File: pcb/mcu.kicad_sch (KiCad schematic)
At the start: 34 parts, among them J1 Conn_01x02_Pin, SW1 SW_SPDT, SW2 SW_Push, SW3 SW_SPDT, U1 TLV1117LV33DCYR, U2 W25Q64JVSSIQ_C179171, U3 STM32H750VBTx, Y1 25 MHz

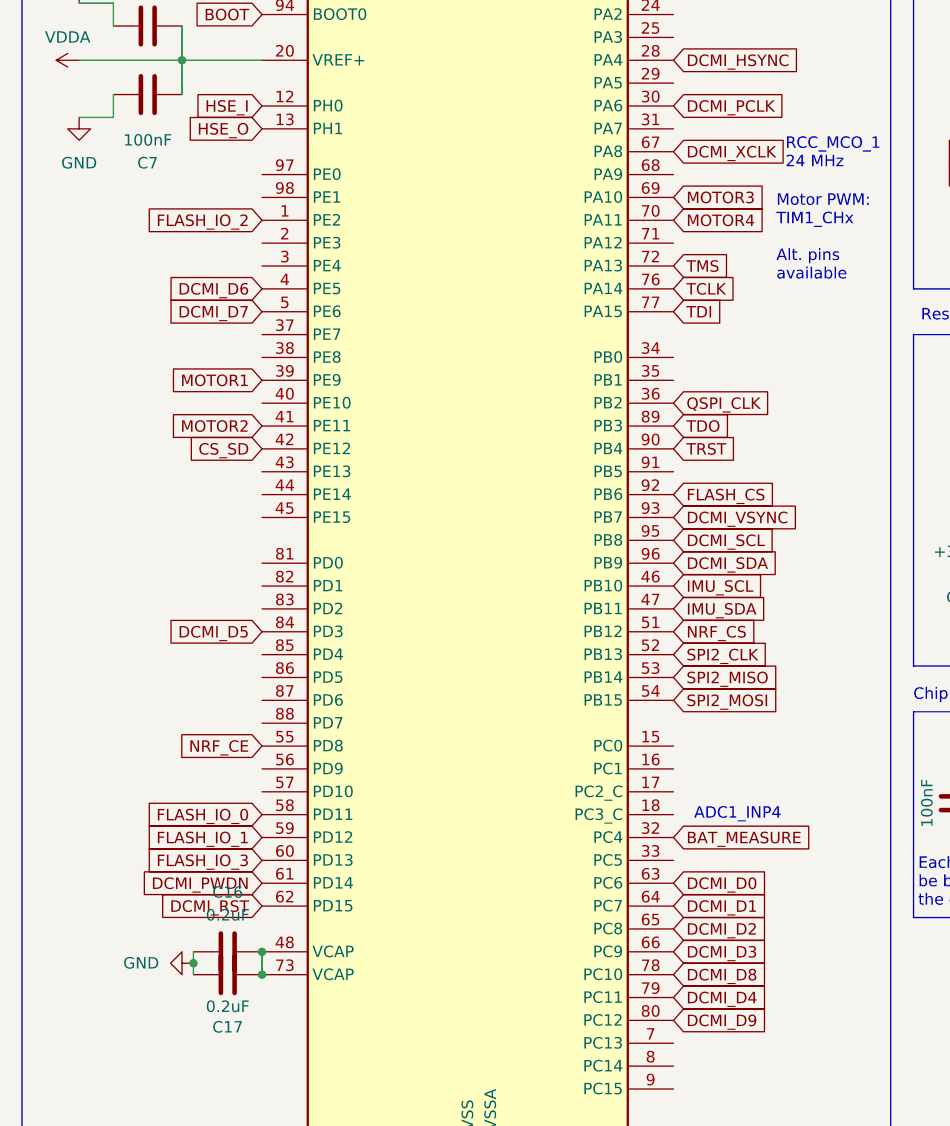
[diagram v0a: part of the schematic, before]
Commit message: [pcb] more routing
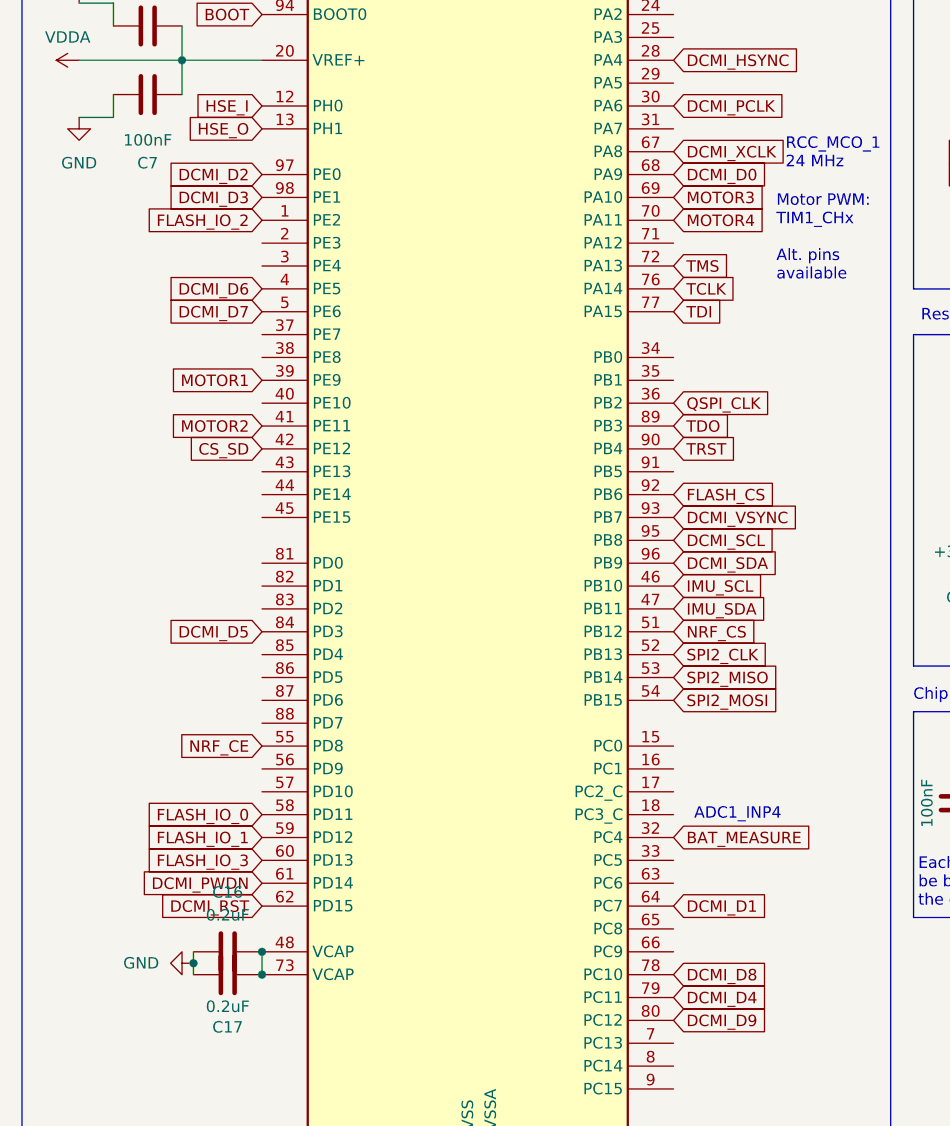
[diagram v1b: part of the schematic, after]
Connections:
- net DCMI_D0: now also U3.68 (PA9); no longer U3.63 (PC6)
- net DCMI_D2: now also U3.97 (PE0); no longer U3.65 (PC8)
- net DCMI_D3: now also U3.98 (PE1); no longer U3.66 (PC9)
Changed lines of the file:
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@@
+		)
+	)
+	(global_label "DCMI_D0"
+		(shape input)
+		(at 87.63 68.58 0)
+		(fields_autoplaced yes)
+		(effects
+			(font
+				(size 1.27 1.27)
+			)
+			(justify left)
+		)
+		(property "Intersheetrefs" "${INTERSHEET_REFS}"
+			(at 98.6585 68.58 0)
+			(effects
+				(font
+					(size 1.27 1.27)
+				)
+				(justify left)
+				(hide yes)
+			)
 		)
 	)
@@
 		)
 	)
+	(global_label "DCMI_PCLK"
+		(shape input)
+		(at 87.63 60.96 0)
+		(fields_autoplaced yes)
+		(effects
+			(font
+				(size 1.27 1.27)
+			)
+			(justify left)
+		)
+		(property "Intersheetrefs" "${INTERSHEET_REFS}"
+			(at 101.0171 60.96 0)
+			(effects
+				(font
+					(size 1.27 1.27)
+				)
+				(justify left)
+				(hide yes)
+			)
+		)
+	)
+	(global_label "BOOT"
+		(shape input)
+		(at 41.91 50.8 180)
+		(fields_autoplaced yes)
+		(effects
+			(font
+				(size 1.27 1.27)
+			)
+			(justify right)
+		)
+		(property "Intersheetrefs" "${INTERSHEET_REFS}"
+			(at 34.0262 50.8 0)
+			(effects
+				(font
+					(size 1.27 1.27)
+				)
+				(justify right)
+				(hide yes)
+			)
+		)
+	)
 	(global_label "DCMI_D2"
 		(shape input)
-		(at 87.63 152.4 0)
-		(fields_autoplaced yes)
-		(effects
-			(font
-				(size 1.27 1.27)
-			)
-			(justify left)
-		)
-		(property "Intersheetrefs" "${INTERSHEET_REFS}"
-			(at 98.6585 152.4 0)
-			(effects
-				(font
-					(size 1.27 1.27)
-				)
-				(justify left)
-				(hide yes)
-			)
-		)
-	)
-	(global_label "DCMI_PCLK"
-		(shape input)
-		(at 87.63 60.96 0)
-		(fields_autoplaced yes)
-		(effects
-			(font
-				(size 1.27 1.27)
-			)
-			(justify left)
-		)
-		(property "Intersheetrefs" "${INTERSHEET_REFS}"
-			(at 101.0171 60.96 0)
-			(effects
-				(font
-					(size 1.27 1.27)
-				)
-				(justify left)
-				(hide yes)
-			)
-		)
-	)
-	(global_label "BOOT"
-		(shape input)
-		(at 41.91 50.8 180)
-		(fields_autoplaced yes)
-		(effects
-			(font
-				(size 1.27 1.27)
-			)
-			(justify right)
-		)
-		(property "Intersheetrefs" "${INTERSHEET_REFS}"
-			(at 34.0262 50.8 0)
+		(at 41.91 68.58 180)
+		(fields_autoplaced yes)
+		(effects
+			(font
+				(size 1.27 1.27)
+			)
+			(justify right)
+		)
+		(property "Intersheetrefs" "${INTERSHEET_REFS}"
+			(at 30.8815 68.58 0)
 			(effects
 				(font
@@
 		)
 	)
+	(global_label "DCMI_D3"
+		(shape input)
+		(at 41.91 71.12 180)
+		(fields_autoplaced yes)
+		(effects
+			(font
+				(size 1.27 1.27)
+			)
+			(justify right)
+		)
+		(property "Intersheetrefs" "${INTERSHEET_REFS}"
+			(at 30.8815 71.12 0)
+			(effects
+				(font
+					(size 1.27 1.27)
+				)
+				(justify right)
+				(hide yes)
+			)
+		)
+	)
 	(global_label "DCMI_SDA"
 		(shape input)
@@
 		)
 	)
-	(global_label "DCMI_D0"
-		(shape input)
-		(at 87.63 147.32 0)
-		(fields_autoplaced yes)
-		(effects
-			(font
-				(size 1.27 1.27)
-			)
-			(justify left)
-		)
-		(property "Intersheetrefs" "${INTERSHEET_REFS}"
-			(at 98.6585 147.32 0)
-			(effects
-				(font
-					(size 1.27 1.27)
-				)
-				(justify left)
-				(hide yes)
-			)
-		)
-	)
 	(global_label "DCMI_HSYNC"
 		(shape input)
@@
 			(effects
 				(font
-					(size 1.27 1.27)
-				)
-				(justify left)
-				(hide yes)
-			)
-		)
-	)
-	(global_label "DCMI_D3"
-		(shape input)
-		(at 87.63 154.94 0)
-		(fields_autoplaced yes)
-		(effects
-			(font
-				(size 1.27 1.27)
-			)
-			(justify left)
-		)
-		(property "Intersheetrefs" "${INTERSHEET_REFS}"
-			(at 98.6585 154.94 0)
-			(effects
-				(font
